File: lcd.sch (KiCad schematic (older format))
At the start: 16 parts, among them J12 Conn_01x14_Female

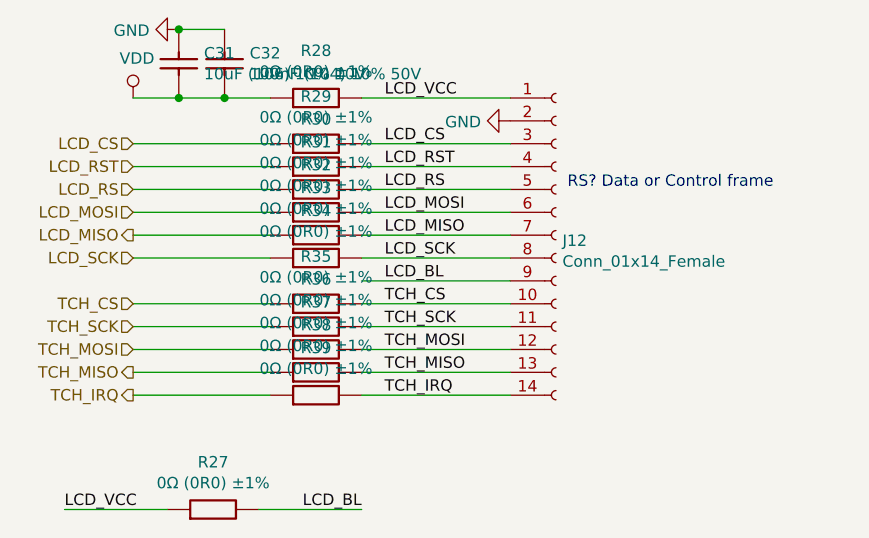
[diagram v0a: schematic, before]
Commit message: 20191114
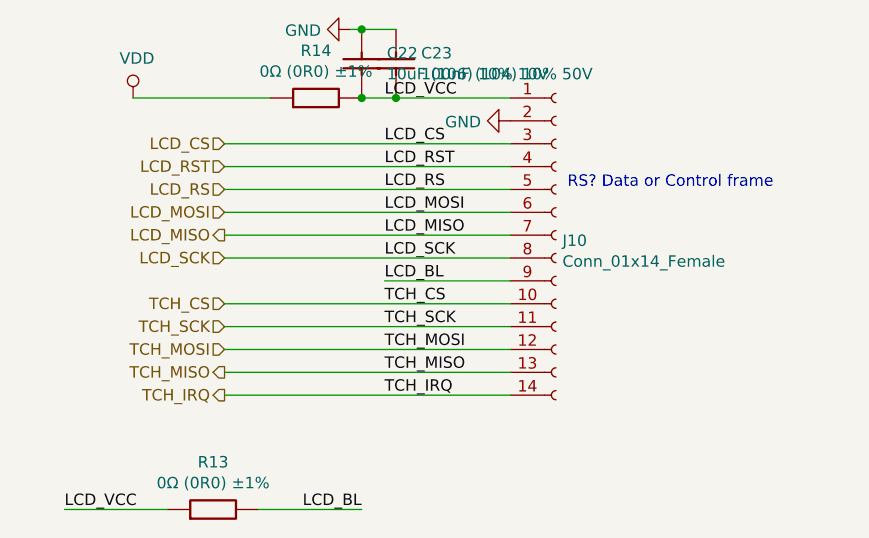
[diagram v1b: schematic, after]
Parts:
- removed R29, R30, R31, R32, R33, R34, R35, R36, R37, R38, R39: 0603_0Ω__0R0_1%, lc_lib:0603_R, symbol lc_RES:0603_0Ω__0R0_1%
- renumbered C31 to C22, C32 to C23, J12 to J10, R27 to R13, R28 to R14
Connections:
- net LCD_VCC: now also C22.2, C23.2
- net VDD: no longer C22.2, C23.2
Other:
- moved on the sheet: C22, C23
